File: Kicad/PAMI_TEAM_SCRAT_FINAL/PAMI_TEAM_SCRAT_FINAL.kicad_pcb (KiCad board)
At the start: 2 copper layers, 60 x 90 mm, 61 parts, among them J1 ALIM, J2 TOF, J3 IR, J4 M1, J5 M2, J6 XL320, SW1 BTN1, SW2 BTN2, SW3 BTN3, SW4 RESET, U1 STM32H573RITx, U2 STLINK-V3MODS, U3 WE-DC-DC-5V, U4 AZ1117CH2-3.3, U5 TB6612FNG, Y1 Crystal

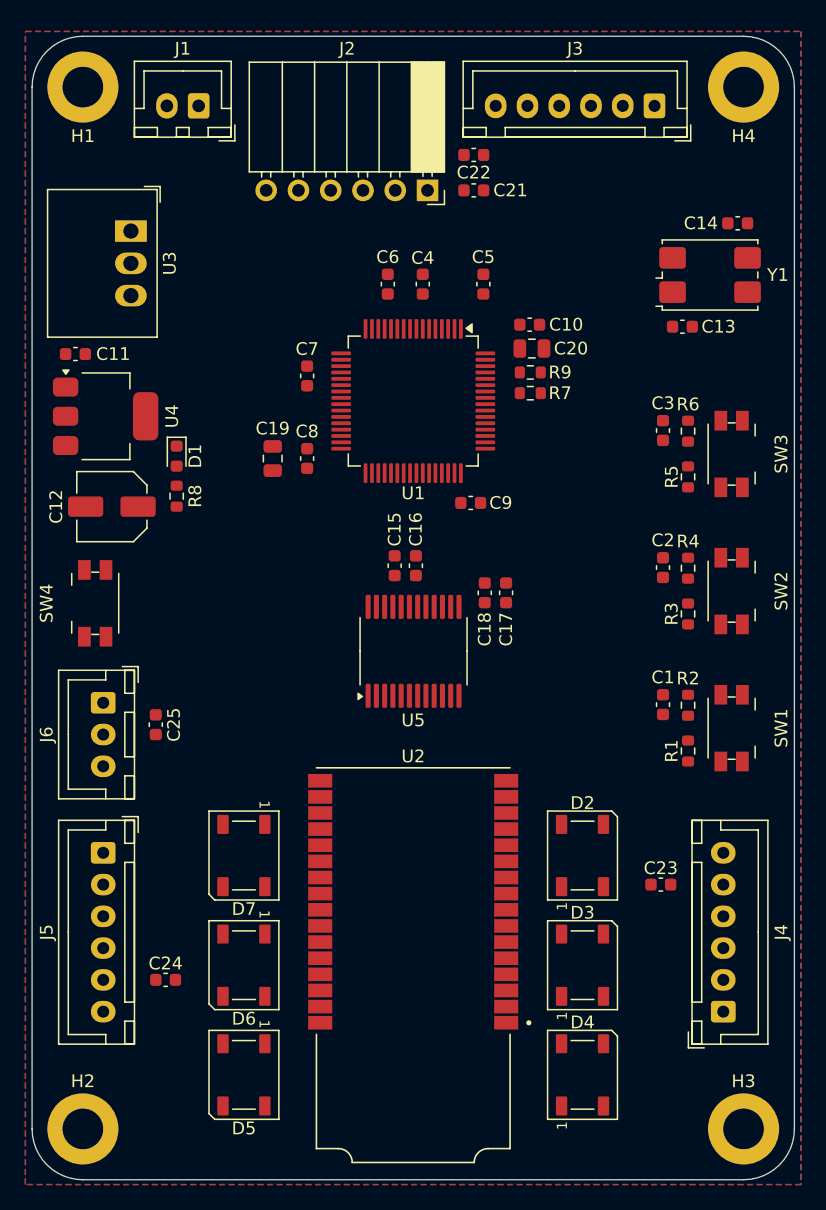
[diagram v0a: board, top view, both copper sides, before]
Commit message: pcb termine
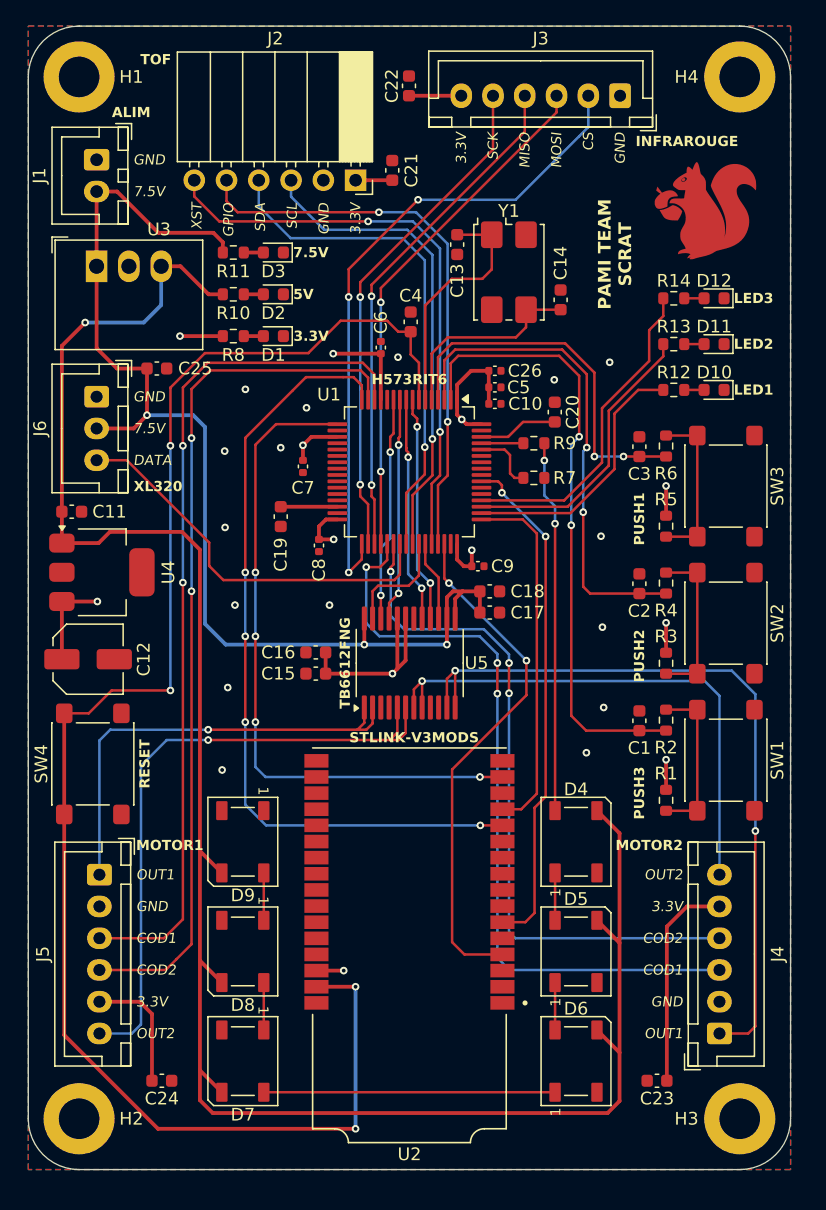
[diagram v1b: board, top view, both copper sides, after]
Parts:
- added C26: 4u7, Capacitor_SMD:C_0402_1005Metric, F.Cu at (147.7, 69.1)
- added D10: LED, LED_SMD:LED_0603_1608Metric, F.Cu at (165.0, 70.6)
- added D11: LED, LED_SMD:LED_0603_1608Metric, F.Cu at (165.0, 67.0)
- added D12: LED, LED_SMD:LED_0603_1608Metric, F.Cu at (165.0, 63.4)
- added D2: LED, LED_SMD:LED_0603_1608Metric, F.Cu at (130.3, 63.1)
- added D3: LED, LED_SMD:LED_0603_1608Metric, F.Cu at (130.3, 59.8)
- added G***: LOGO, LOGOS:ecureuil_8mm, F.Cu at (164.3, 56.5)
- added R10: 3k3, Resistor_SMD:R_0603_1608Metric, F.Cu at (127.1, 63.1)
- added R11: 5k8, Resistor_SMD:R_0603_1608Metric, F.Cu at (127.1, 59.8)
- added R12: 1k6, Resistor_SMD:R_0603_1608Metric, F.Cu at (161.8, 70.6)
- added R13: 1k6, Resistor_SMD:R_0603_1608Metric, F.Cu at (161.8, 67.0)
- added R14: 1k6, Resistor_SMD:R_0603_1608Metric, F.Cu at (161.8, 63.4)
- C10, C5, C6, C7, C8, C9: footprint Capacitor_SMD:C_0603_1608Metric -> Capacitor_SMD:C_0402_1005Metric
- C19, C20: value 22u -> 2u2; footprint Capacitor_SMD:C_0805_2012Metric -> Capacitor_SMD:C_0603_1608Metric
- R8: value 510 -> 1k6
- SW1, SW2, SW3, SW4: footprint Button_Switch_SMD:Panasonic_EVQPUJ_EVQPUA -> Button_Switch_SMD:SW_SPST_PTS645Sx43SMTR92
- U3: value WE-DC-DC-5V -> 173010578
- moved C25 28.0 mm to (121.1, 69.0), turned to 180 degrees
- moved J6 24.1 mm to (116.4, 71.2)
- moved C13 18.9 mm to (144.8, 59.2), turned to -90 degrees
- moved Y1 15.8 mm to (148.8, 61.4), turned to -90 degrees
- moved C23 15.4 mm to (160.5, 125.0)
- moved C14 15.2 mm to (152.9, 63.5), turned to -90 degrees
- moved R8 13.4 mm to (127.1, 66.4), turned to 0 degrees
- moved SW4 12.6 mm to (116.1, 100.1)
- moved C11 12.4 mm to (114.4, 80.2)
- moved U4 12.3 mm to (116.8, 85.0)
- moved C12 12.2 mm to (115.7, 91.8), turned to 0 degrees
- moved D1 12.1 mm to (130.3, 66.4), turned to 180 degrees
- moved C15 10.5 mm to (133.6, 93.0), turned to 180 degrees
- moved C16 10.4 mm to (133.6, 91.3), turned to 180 degrees
- moved J1 9.08 mm to (116.4, 52.5), turned to -90 degrees
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- renumbered D2 to D4, D3 to D5, D4 to D6, D5 to D7, D6 to D8, D7 to D9
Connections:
- C11 pad 1: Net-(U3-OUT) -> +5V
- D4 pad 3: +3.3V -> +5V
- D5 pad 3: +3.3V -> +5V
- D6 pad 3: +3.3V -> +5V
- D7 pad 3: +3.3V -> +5V
- D8 pad 3: +3.3V -> +5V
- D9 pad 3: +3.3V -> +5V
- J4 pad 1: /A_O1 -> /B_O1
- J4 pad 3: A_ENC1 -> B_ENC1
- J4 pad 4: A_ENC2 -> B_ENC2
- J4 pad 6: /A_O2 -> /B_O2
- J5 pad 1: /B_O1 -> /A_O1
- J5 pad 3: B_ENC1 -> A_ENC1
- J5 pad 4: B_ENC2 -> A_ENC2
- J5 pad 6: /B_O2 -> /A_O2
- U1 pad 10: B_IN1 -> A_IN1
- U1 pad 11: B_IN2 -> A_IN2
- U1 pad 44: GPIO -> XST
- U1 pad 45: XST -> GPIO
- U1 pad 50: unconnected-(U1-PA15(JTDI)-Pad50) -> Net-(U1-PA15(JTDI))
- U1 pad 51: unconnected-(U1-PC10-Pad51) -> Net-(U1-PC10)
- U1 pad 52: unconnected-(U1-PC11-Pad52) -> Net-(U1-PC11)
- U1 pad 8: A_IN1 -> B_IN2
- U1 pad 9: A_IN2 -> B_IN1
- U3 pad 3: Net-(U3-OUT) -> +5V
- U4 pad 1: Net-(U3-OUT) -> +5V
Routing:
- net +5V: track 0.00 -> 158.4 mm, vias 0 -> 1
- net /MCU STM32/NRST: track 0.00 -> 125.6 mm, vias 0 -> 4
- net +3.3V: track 0.00 -> 98.7 mm, vias 0 -> 12
- net +7.5V: track 0.00 -> 90.2 mm, vias 0 -> 3
- net A_ENC2: track 0.00 -> 68.3 mm, vias 0 -> 2
- net A_ENC1: track 0.00 -> 67.3 mm, vias 0 -> 2
- net /MCU STM32/UART_TX: track 0.00 -> 62.3 mm, vias 0 -> 4
- net B_ENC1: track 0.00 -> 60.7 mm, vias 0 -> 3
- net /B_O1: track 0.00 -> 59.7 mm, vias 0 -> 2
- net B_ENC2: track 0.00 -> 54.9 mm, vias 0 -> 3
- net SPI_CS: track 0.00 -> 52.5 mm, vias 0 -> 3
- net /MCU STM32/UART_RX: track 0.00 -> 52.2 mm, vias 0 -> 4
- net /A_O2: track 0.00 -> 50.6 mm, vias 0 -> 1
- net BTN1: track 0.00 -> 48.8 mm, vias 0 -> 2
- net XST: track 0.00 -> 45.8 mm, vias 0 -> 2
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- added copper zone on In2.Cu, net +3.3V
- added copper zone on In1.Cu, net B_IN2
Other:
- copper layers 2 -> 4
- board text added: "3.3V"
- board text added: "5V"
- board text added: "7.5V"
- board text added: "ALIM"
- board text added: "COD1"
- board text added: "COD2"
- board text added: "CS"
- board text added: "DATA"
- board text added: "GND"
- board text added: "GPIO"
- board text added: "H573RIT6"
- board text added: "INFRAROUGE"
- board text added: "LED1"
- board text added: "LED2"
- board text added: "LED3"
- board text added: "MISO"
- board text added: "MOSI"
- board text added: "MOTOR1"
- board text added: "MOTOR2"
- board text added: "OUT1"
- board text added: "OUT2"
- board text added: "PAMI TEAM SCRAT"
- board text added: "PUSH1"
- board text added: "PUSH2"
- board text added: "PUSH3"
- board text added: "RESET"
- board text added: "SCK"
- board text added: "SCL"
- board text added: "SDA"
- board text added: "STLINK-V3MODS"
- board text added: "TB6612FNG"
- board text added: "TOF"
- board text added: "XL320"
- board text added: "XST"
